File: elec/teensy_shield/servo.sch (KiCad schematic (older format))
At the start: 0 parts

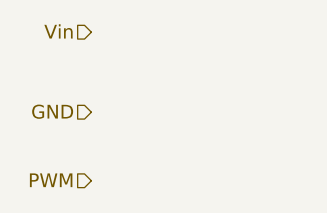
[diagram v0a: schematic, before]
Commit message: Completed new board schematics.
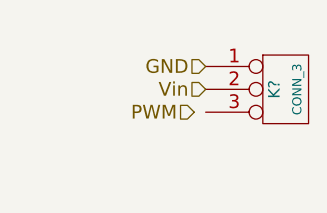
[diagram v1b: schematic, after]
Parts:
- added K?: CONN_3, symbol CONN_3
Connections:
- net GND: now also K?.1 (P1)
- net Vin: now also K?.2 (PM)
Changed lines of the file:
@@
 LIBS:contrib
 LIBS:valves
+LIBS:arduino_shieldsNCL
+LIBS:teensy
+LIBS:pololu
+LIBS:teensy_shield-cache
 EELAYER 24 0
 EELAYER END
 $Descr A4 11693 8268
 encoding utf-8
-Sheet 4 26
+Sheet 5 34
 Title ""
 Date ""
@@
 Comment4 ""
 $EndDescr
-Text HLabel 4400 2850 0    60   Input ~ 0
+Text HLabel 4900 3100 0    60   Input ~ 0
 Vin
-Text HLabel 4400 3200 0    60   Input ~ 0
+Text HLabel 4900 3000 0    60   Input ~ 0
 GND
-Text HLabel 4400 3500 0    60   Input ~ 0
+Text HLabel 4850 3200 0    60   Input ~ 0
 PWM
+$Comp
+L CONN_3 K?
+U 1 1 55E819AD
+P 5250 3100
+F 0 "K?" V 5200 3100 50  0000 C CNN
+F 1 "CONN_3" V 5300 3100 40  0000 C CNN
+F 2 "" H 5250 3100 60  0000 C CNN
+F 3 "" H 5250 3100 60  0000 C CNN
+	1    5250 3100
+	1    0    0    -1
+$EndComp
 $EndSCHEMATC
